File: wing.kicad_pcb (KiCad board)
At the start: 2 copper layers, 198.4 x 102.7 mm, 61 parts, among them J1 pin_array_2x1, U1 DSP310_DEV, U10 DPS310_DEV, U11 DPS310_DEV, U12 DPS310_DEV, U13 DPS310_DEV, U14 DPS310_DEV, U15 DPS310_DEV, U16 DPS310_DEV, U17 DPS310_DEV, U18 DPS310_DEV, U19 DPS310_DEV, U2 DSP310_DEV, U20 DPS310_DEV, U21 DPS310_DEV, U22 DPS310_DEV, U23 DPS310_DEV, U24 DPS310_DEV, U25 DPS310_DEV, U26 DPS310_DEV, U27 DPS310_DEV, U28 DPS310_DEV, U29 DPS310_DEV, U3 DPS310_DEV, U30 DPS310_DEV, U31 DPS310_DEV, U32 DPS310_DEV, U33 DPS310_DEV, U34 DPS310_DEV, U35 DPS310_DEV, U36 DPS310_DEV, U37 DPS310_DEV, U38 DPS310_DEV, U39 DPS310_DEV, U4 DPS310_DEV, U40 DPS310_DEV, U41 DPS310_DEV, U42 DPS310_DEV, U43 DPS310_DEV, U44 DPS310_DEV, U45 DPS310_DEV, U46 DPS310_DEV, U47 DPS310_DEV, U48 DPS310_DEV, U49 DPS310_DEV, U5 DPS310_DEV, U50 DPS310_DEV, U51 DPS310_DEV, U52 DPS310_DEV, U53 teensy3.5, U54 Adafruit_BNO055, U6 DPS310_DEV, U7 DPS310_DEV, U8 DPS310_DEV, U9 DPS310_DEV

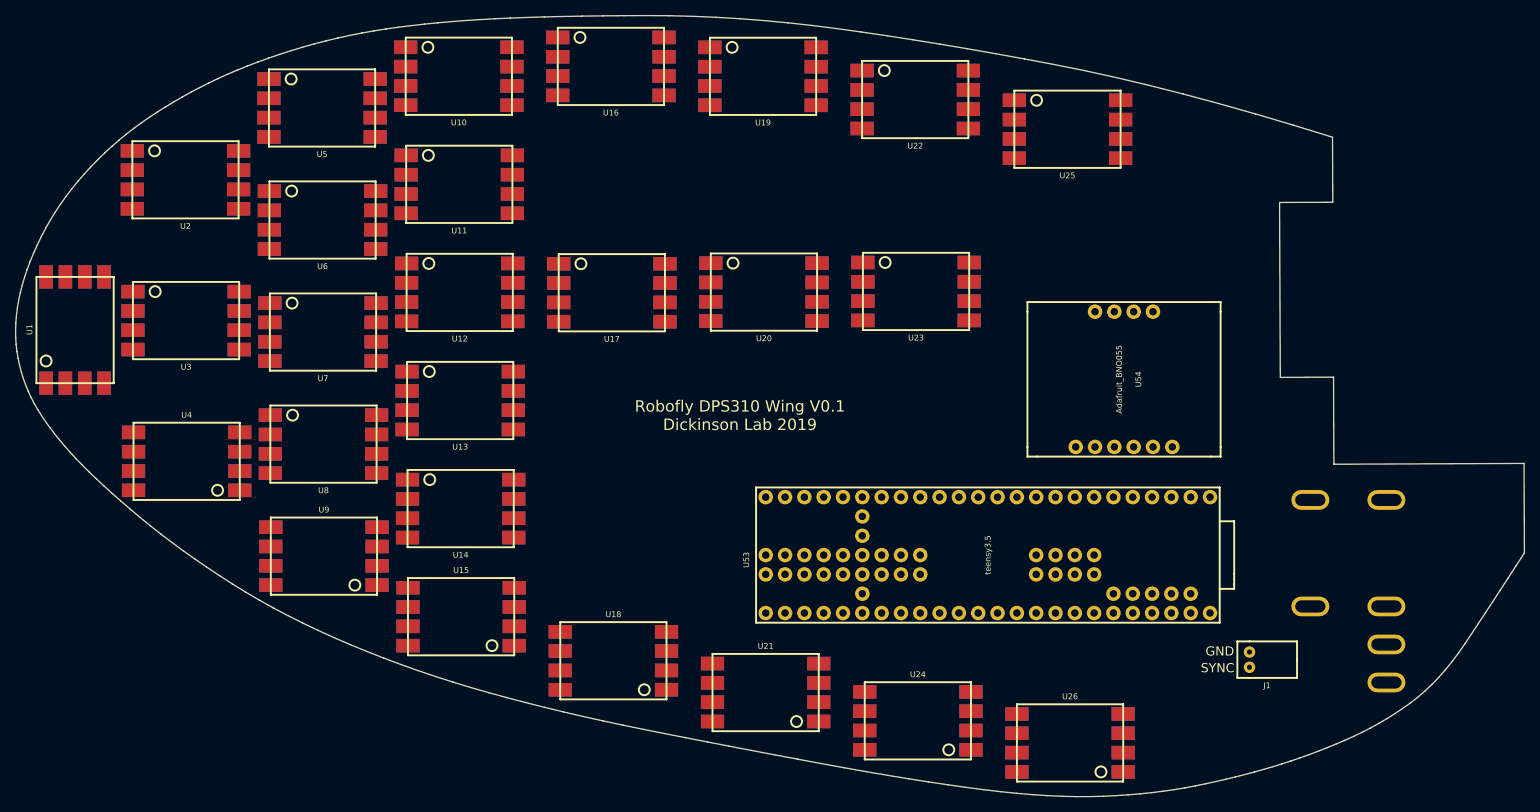
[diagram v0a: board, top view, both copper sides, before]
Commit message: Added readme and images.
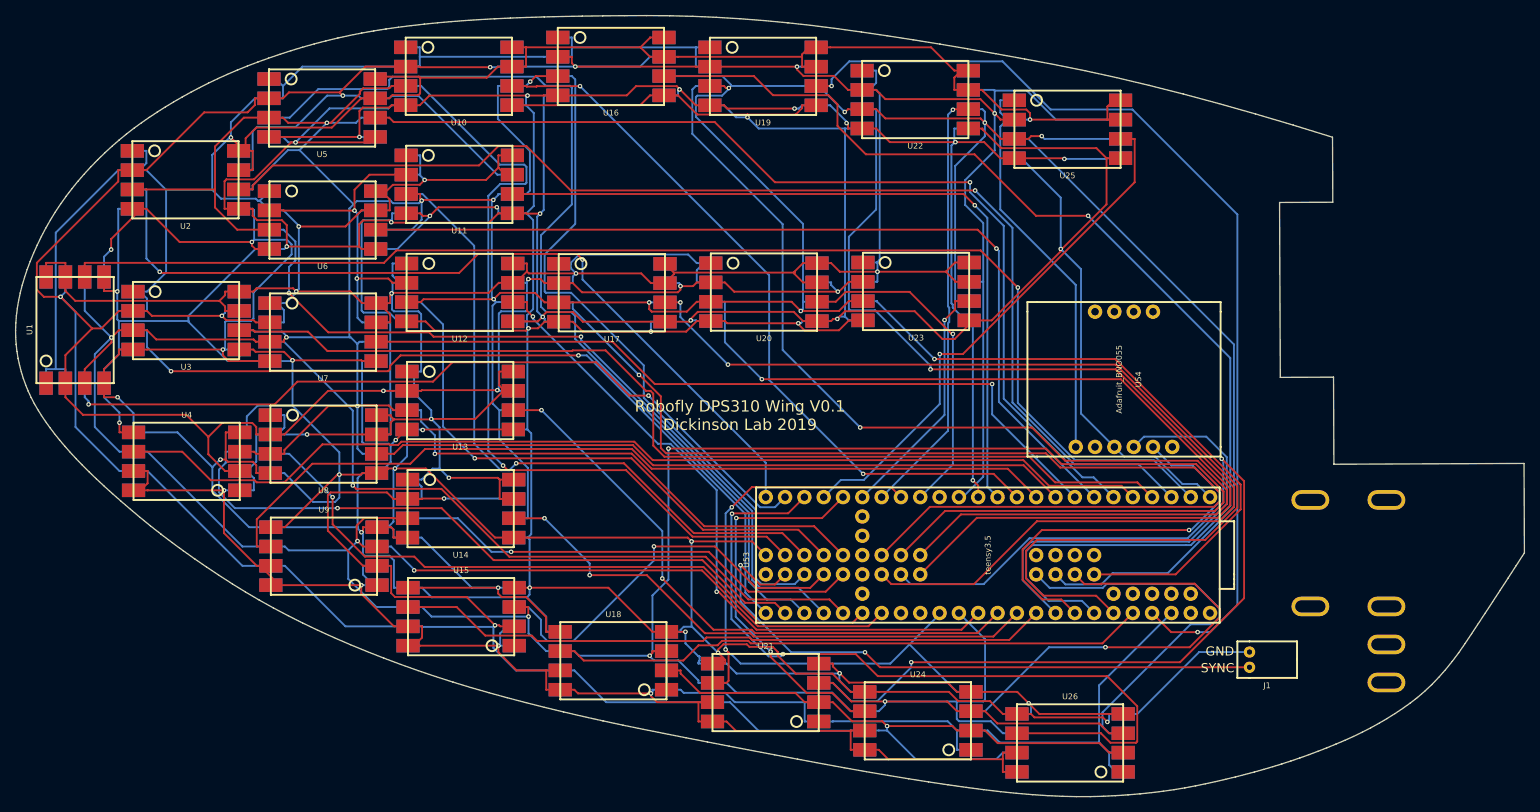
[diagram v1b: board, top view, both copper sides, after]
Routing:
- net /3V3: track 0.00 -> 1084.0 mm, vias 0 -> 15
- net GND: track 0.00 -> 865.0 mm, vias 0 -> 19
- net /MISO: track 0.00 -> 846.5 mm, vias 0 -> 17
- net /SCK: track 0.00 -> 759.1 mm, vias 0 -> 18
- net /MOSI: track 0.00 -> 679.5 mm, vias 0 -> 24
- net /DPS_CS00: track 0.00 -> 170.3 mm, vias 0 -> 1
- net /DPS_CS01: track 0.00 -> 157.9 mm, vias 0 -> 1
- net /DPS_CS15: track 0.00 -> 154.6 mm, vias 0 -> 1
- net /DPS_CS44: track 0.00 -> 152.6 mm, vias 0 -> 1
- net /DPS_CS43: track 0.00 -> 151.4 mm, vias 0 -> 1
- net /DPS_CS42: track 0.00 -> 150.3 mm, vias 0 -> 1
- net /DPS_CS47: track 0.00 -> 143.8 mm, vias 0 -> 1
- net /DPS_CS03: track 0.00 -> 138.4 mm
- net /DPS_CS16: track 0.00 -> 136.4 mm, vias 0 -> 2
- net /DPS_CS46: track 0.00 -> 135.7 mm, vias 0 -> 2
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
